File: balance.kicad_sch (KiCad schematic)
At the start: 24 parts, among them Q10 2N7002, Q5 AO3401A, Q6 AO3401A, Q7 AO3401A, Q8 2N7002, Q9 2N7002

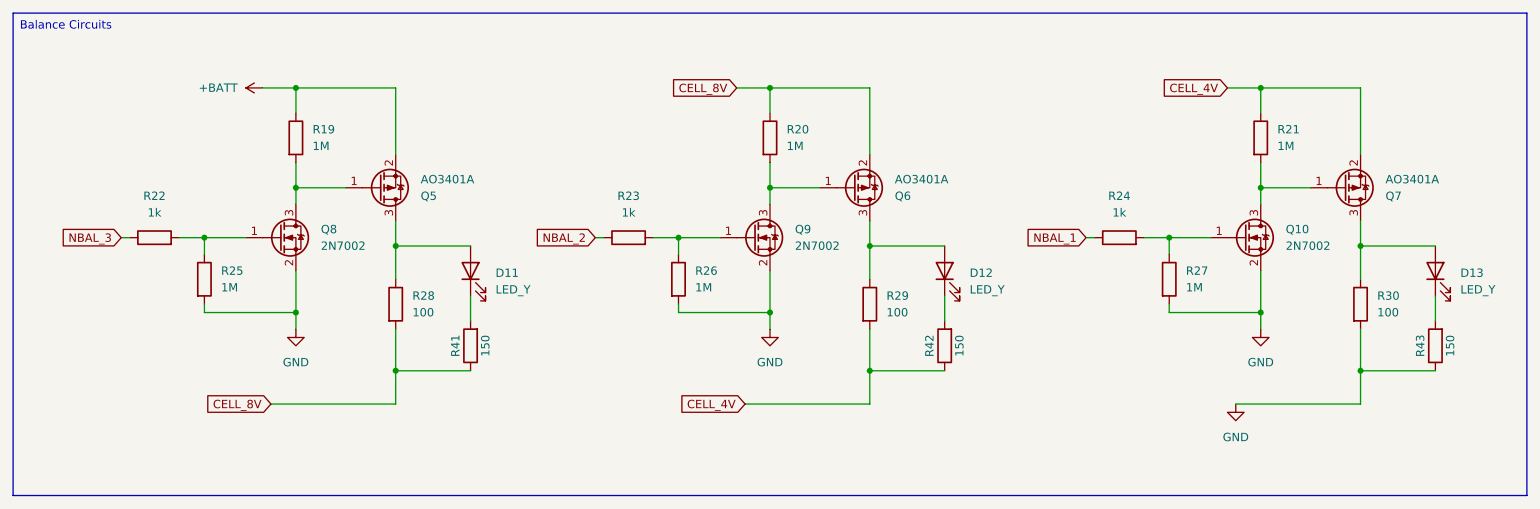
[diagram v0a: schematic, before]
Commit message: Decent pass
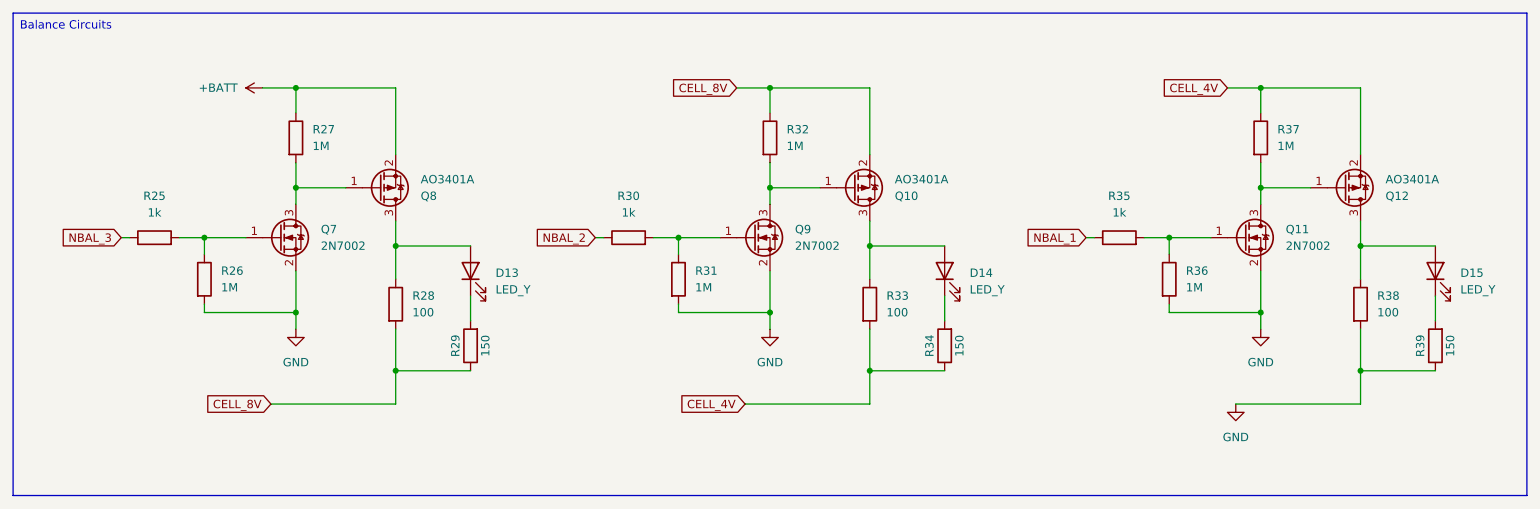
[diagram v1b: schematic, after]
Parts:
- renumbered D11 to D13, D12 to D14, D13 to D15, Q6 to Q10, Q10 to Q11, Q7 to Q12, Q8 to Q7, Q5 to Q8, R22 to R25, R25 to R26, R19 to R27, R41 to R29, R23 to R30, R26 to R31, R20 to R32, R29 to R33, R42 to R34, R24 to R35, R27 to R36, R21 to R37, R30 to R38, R43 to R39
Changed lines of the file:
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@@
 		(dnp no)
 		(fields_autoplaced yes)
-		(property "Reference" "D12"
+		(property "Reference" "D14"
 			(at 184.15 65.0874 90)
 			(effects
@@
 			(project "JPBms2"
 				(path "/d86e471c-a8be-422d-a5d1-5a4699b7b766/220685a5-608c-4c12-9441-6825efcef07c"
-					(reference "D12")
+					(reference "D14")
 					(unit 1)
 				)
@@
 		(dnp no)
 		(fields_autoplaced yes)
-		(property "Reference" "#PWR042"
+		(property "Reference" "#PWR048"
 			(at 80.01 36.83 0)
 			(effects
@@
 			(project "JPBms2"
 				(path "/d86e471c-a8be-422d-a5d1-5a4699b7b766/220685a5-608c-4c12-9441-6825efcef07c"
-					(reference "#PWR042")
+					(reference "#PWR048")
 					(unit 1)
 				)
@@
 		(dnp no)
 		(fields_autoplaced yes)
-		(property "Reference" "R25"
+		(property "Reference" "R26"
 			(at 69.85 64.7699 0)
 			(effects
@@
 			(project "JPBms2"
 				(path "/d86e471c-a8be-422d-a5d1-5a4699b7b766/220685a5-608c-4c12-9441-6825efcef07c"
-					(reference "R25")
+					(reference "R26")
 					(unit 1)
 				)
@@
 		(dnp no)
 		(fields_autoplaced yes)
-		(property "Reference" "R27"
+		(property "Reference" "R36"
 			(at 217.17 64.7699 0)
 			(effects
@@
 			(project "JPBms2"
 				(path "/d86e471c-a8be-422d-a5d1-5a4699b7b766/220685a5-608c-4c12-9441-6825efcef07c"
-					(reference "R27")
+					(reference "R36")
 					(unit 1)
 				)
@@
 		(dnp no)
 		(fields_autoplaced yes)
-		(property "Reference" "R24"
+		(property "Reference" "R35"
 			(at 207.01 53.34 90)
 			(effects
@@
 			(project "JPBms2"
 				(path "/d86e471c-a8be-422d-a5d1-5a4699b7b766/220685a5-608c-4c12-9441-6825efcef07c"
-					(reference "R24")
+					(reference "R35")
 					(unit 1)
 				)
@@
 		(on_board yes)
 		(dnp no)
-		(property "Reference" "R42"
+		(property "Reference" "R34"
 			(at 178.054 76.2 90)
 			(effects
@@
 			(project "JPBms2"
 				(path "/d86e471c-a8be-422d-a5d1-5a4699b7b766/220685a5-608c-4c12-9441-6825efcef07c"
-					(reference "R42")
+					(reference "R34")
 					(unit 1)
 				)
@@
 		(on_board yes)
 		(dnp no)
-		(property "Reference" "R43"
+		(property "Reference" "R39"
 			(at 252.984 76.2 90)
 			(effects
@@
 			(project "JPBms2"
 				(path "/d86e471c-a8be-422d-a5d1-5a4699b7b766/220685a5-608c-4c12-9441-6825efcef07c"
-					(reference "R43")
+					(reference "R39")
 					(unit 1)
 				)
@@
 		(dnp no)
 		(fields_autoplaced yes)
-		(property "Reference" "Q8"
+		(property "Reference" "Q7"
 			(at 85.09 58.4199 0)
 			(effects
@@
 			(project "JPBms2"
 				(path "/d86e471c-a8be-422d-a5d1-5a4699b7b766/220685a5-608c-4c12-9441-6825efcef07c"
-					(reference "Q8")
+					(reference "Q7")
 					(unit 1)
 				)
@@
 		(dnp no)
 		(fields_autoplaced yes)
-		(property "Reference" "R26"
+		(property "Reference" "R31"
 			(at 142.24 64.7699 0)
 			(effects
@@
 			(project "JPBms2"
 				(path "/d86e471c-a8be-422d-a5d1-5a4699b7b766/220685a5-608c-4c12-9441-6825efcef07c"
-					(reference "R26")
+					(reference "R31")
 					(unit 1)
 				)
@@
 		(on_board yes)
 		(dnp no)
-		(property "Reference" "R41"
+		(property "Reference" "R29"
 			(at 105.664 76.2 90)
 			(effects
@@
 			(project "JPBms2"
 				(path "/d86e471c-a8be-422d-a5d1-5a4699b7b766/220685a5-608c-4c12-9441-6825efcef07c"
-					(reference "R41")
+					(reference "R29")
 					(unit 1)
 				)
@@
 		(dnp no)
 		(fields_autoplaced yes)
-		(property "Reference" "R20"
+		(property "Reference" "R32"
 			(at 156.21 43.1799 0)
 			(effects
@@
 			(project "JPBms2"
 				(path "/d86e471c-a8be-422d-a5d1-5a4699b7b766/220685a5-608c-4c12-9441-6825efcef07c"
-					(reference "R20")
+					(reference "R32")
 					(unit 1)
 				)
@@
 		(dnp no)
 		(fields_autoplaced yes)
-		(property "Reference" "#PWR046"
+		(property "Reference" "#PWR051"
 			(at 224.79 91.44 0)
 			(effects
@@
 			(project "JPBms2"
 				(path "/d86e471c-a8be-422d-a5d1-5a4699b7b766/220685a5-608c-4c12-9441-6825efcef07c"
-					(reference "#PWR046")
+					(reference "#PWR051")
 					(unit 1)
 				)
@@
 		(dnp no)
 		(fields_autoplaced yes)
-		(property "Reference" "Q10"
+		(property "Reference" "Q11"
 			(at 232.41 58.4199 0)
 			(effects
@@
 			(project "JPBms2"
 				(path "/d86e471c-a8be-422d-a5d1-5a4699b7b766/220685a5-608c-4c12-9441-6825efcef07c"
-					(reference "Q10")
+					(reference "Q11")
 					(unit 1)
 				)
@@
 		(dnp no)
 		(fields_autoplaced yes)
-		(property "Reference" "R30"
+		(property "Reference" "R38"
 			(at 246.38 68.5799 0)
 			(effects
@@
 			(project "JPBms2"
 				(path "/d86e471c-a8be-422d-a5d1-5a4699b7b766/220685a5-608c-4c12-9441-6825efcef07c"
-					(reference "R30")
+					(reference "R38")
 					(unit 1)
 				)
@@
 		(dnp no)
 		(fields_autoplaced yes)
-		(property "Reference" "#PWR045"
+		(property "Reference" "#PWR052"
 			(at 228.6 80.01 0)
 			(effects
@@
 			(project "JPBms2"
 				(path "/d86e471c-a8be-422d-a5d1-5a4699b7b766/220685a5-608c-4c12-9441-6825efcef07c"
-					(reference "#PWR045")
+					(reference "#PWR052")
 					(unit 1)
 				)
@@
 		(dnp no)
 		(fields_autoplaced yes)
-		(property "Reference" "R19"
+		(property "Reference" "R27"
 			(at 83.82 43.1799 0)
 			(effects
@@
 			(project "JPBms2"
 				(path "/d86e471c-a8be-422d-a5d1-5a4699b7b766/220685a5-608c-4c12-9441-6825efcef07c"
-					(reference "R19")
+					(reference "R27")
 					(unit 1)
 				)
@@
 		(dnp no)
 		(fields_autoplaced yes)
-		(property "Reference" "R23"
+		(property "Reference" "R30"
 			(at 132.08 53.34 90)
 			(effects
@@
 			(project "JPBms2"
 				(path "/d86e471c-a8be-422d-a5d1-5a4699b7b766/220685a5-608c-4c12-9441-6825efcef07c"
-					(reference "R23")
+					(reference "R30")
 					(unit 1)
 				)
@@
 		(dnp no)
 		(fields_autoplaced yes)
-		(property "Reference" "D11"
+		(property "Reference" "D13"
 			(at 111.76 65.0874 90)
 			(effects
@@
 			(project "JPBms2"
 				(path "/d86e471c-a8be-422d-a5d1-5a4699b7b766/220685a5-608c-4c12-9441-6825efcef07c"
-					(reference "D11")
+					(reference "D13")
 					(unit 1)
 				)
@@
 		(dnp no)
 		(fields_autoplaced yes)
-		(property "Reference" "R22"
+		(property "Reference" "R25"
 			(at 59.69 53.34 90)
 			(effects
@@
 			(project "JPBms2"
 				(path "/d86e471c-a8be-422d-a5d1-5a4699b7b766/220685a5-608c-4c12-9441-6825efcef07c"
-					(reference "R22")
+					(reference "R25")
 					(unit 1)
 				)
@@
 		(dnp no)
 		(fields_autoplaced yes)
-		(property "Reference" "R29"
+		(property "Reference" "R33"
 			(at 171.45 68.5799 0)
 			(effects
@@
 			(project "JPBms2"
 				(path "/d86e471c-a8be-422d-a5d1-5a4699b7b766/220685a5-608c-4c12-9441-6825efcef07c"
-					(reference "R29")
+					(reference "R33")
 					(unit 1)
 				)
@@
 		(on_board yes)
 		(dnp no)
-		(property "Reference" "Q5"
+		(property "Reference" "Q8"
 			(at 100.33 53.3401 0)
 			(effects
@@
 			(project "JPBms2"
 				(path "/d86e471c-a8be-422d-a5d1-5a4699b7b766/220685a5-608c-4c12-9441-6825efcef07c"
-					(reference "Q5")
+					(reference "Q8")
 					(unit 1)
 				)
@@
 		(on_board yes)
 		(dnp no)
-		(property "Reference" "Q6"
+		(property "Reference" "Q10"
 			(at 172.72 53.3401 0)
 			(effects
@@
 			(project "JPBms2"
 				(path "/d86e471c-a8be-422d-a5d1-5a4699b7b766/220685a5-608c-4c12-9441-6825efcef07c"
-					(reference "Q6")
+					(reference "Q10")
 					(unit 1)
 				)
@@
 		(dnp no)
 		(fields_autoplaced yes)
-		(property "Reference" "#PWR043"
+		(property "Reference" "#PWR049"
 			(at 81.28 80.01 0)
 			(effects
@@
 			(project "JPBms2"
 				(path "/d86e471c-a8be-422d-a5d1-5a4699b7b766/220685a5-608c-4c12-9441-6825efcef07c"
-					(reference "#PWR043")
+					(reference "#PWR049")
 					(unit 1)
 				)
@@
 		(on_board yes)
 		(dnp no)
-		(property "Reference" "Q7"
+		(property "Reference" "Q12"
 			(at 247.65 53.3401 0)
 			(effects
@@
 			(project "JPBms2"
 				(path "/d86e471c-a8be-422d-a5d1-5a4699b7b766/220685a5-608c-4c12-9441-6825efcef07c"
-					(reference "Q7")
+					(reference "Q12")
 					(unit 1)
 				)
@@
 		(dnp no)
 		(fields_autoplaced yes)
-		(property "Reference" "#PWR044"
+		(property "Reference" "#PWR050"
 			(at 153.67 80.01 0)
 			(effects
@@
 			(project "JPBms2"
 				(path "/d86e471c-a8be-422d-a5d1-5a4699b7b766/220685a5-608c-4c12-9441-6825efcef07c"
-					(reference "#PWR044")
+					(reference "#PWR050")
 					(unit 1)
 				)
@@
 		(dnp no)
 		(fields_autoplaced yes)
-		(property "Reference" "D13"
+		(property "Reference" "D15"
 			(at 259.08 65.0874 90)
 			(effects
@@
 			(project "JPBms2"
 				(path "/d86e471c-a8be-422d-a5d1-5a4699b7b766/220685a5-608c-4c12-9441-6825efcef07c"
-					(reference "D13")
+					(reference "D15")
 					(unit 1)
 				)
@@
 		(dnp no)
 		(fields_autoplaced yes)
-		(property "Reference" "R21"
+		(property "Reference" "R37"
 			(at 231.14 43.1799 0)
 			(effects
@@
 			(project "JPBms2"
 				(path "/d86e471c-a8be-422d-a5d1-5a4699b7b766/220685a5-608c-4c12-9441-6825efcef07c"
-					(reference "R21")
-					(unit 1)
-				)
+					(reference "R37")
+					(unit 1)
+				)

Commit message: Routing pt1
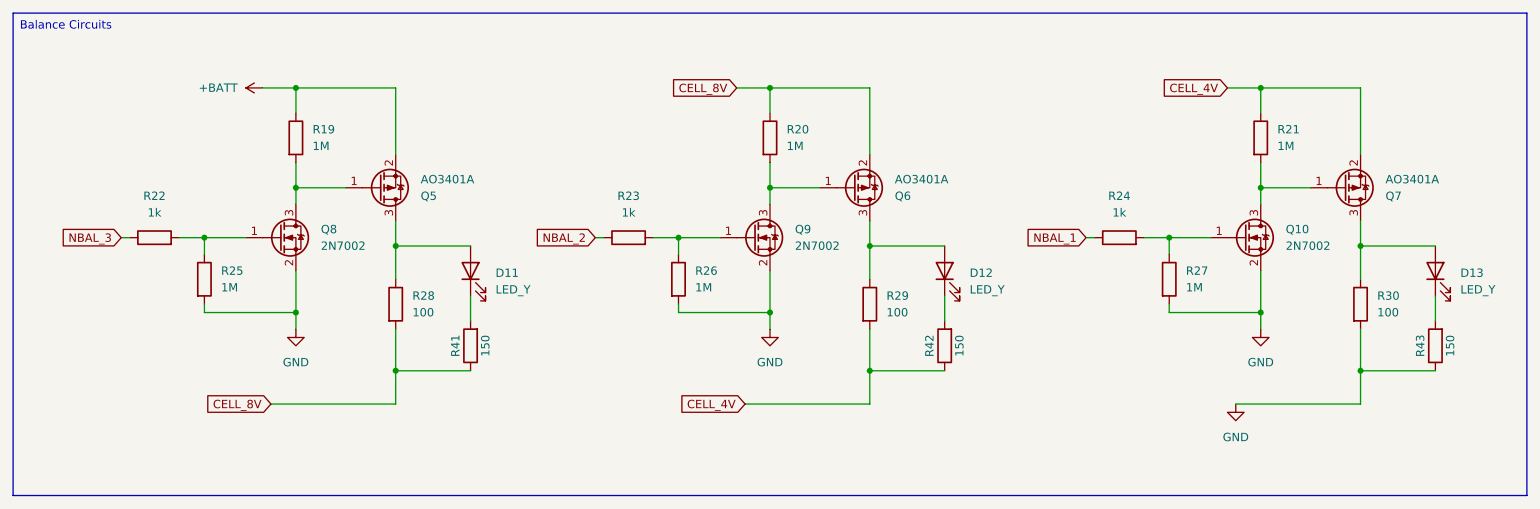
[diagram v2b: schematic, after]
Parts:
- renumbered D13 to D11, D14 to D12, D15 to D13, Q11 to Q10, Q8 to Q5, Q10 to Q6, Q12 to Q7, Q7 to Q8, R27 to R19, R32 to R20, R37 to R21, R25 to R22, R30 to R23, R35 to R24, R26 to R25, R31 to R26, R36 to R27, R33 to R29, R38 to R30, R29 to R41, R34 to R42, R39 to R43
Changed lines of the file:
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@@
 		(dnp no)
 		(fields_autoplaced yes)
-		(property "Reference" "D14"
+		(property "Reference" "D12"
 			(at 184.15 65.0874 90)
 			(effects
@@
 			(project "JPBms2"
 				(path "/d86e471c-a8be-422d-a5d1-5a4699b7b766/220685a5-608c-4c12-9441-6825efcef07c"
-					(reference "D14")
+					(reference "D12")
 					(unit 1)
 				)
@@
 		(dnp no)
 		(fields_autoplaced yes)
-		(property "Reference" "#PWR048"
+		(property "Reference" "#PWR042"
 			(at 80.01 36.83 0)
 			(effects
@@
 			(project "JPBms2"
 				(path "/d86e471c-a8be-422d-a5d1-5a4699b7b766/220685a5-608c-4c12-9441-6825efcef07c"
-					(reference "#PWR048")
+					(reference "#PWR042")
 					(unit 1)
 				)
@@
 		(dnp no)
 		(fields_autoplaced yes)
-		(property "Reference" "R26"
+		(property "Reference" "R25"
 			(at 69.85 64.7699 0)
 			(effects
@@
 			(project "JPBms2"
 				(path "/d86e471c-a8be-422d-a5d1-5a4699b7b766/220685a5-608c-4c12-9441-6825efcef07c"
-					(reference "R26")
+					(reference "R25")
 					(unit 1)
 				)
@@
 		(dnp no)
 		(fields_autoplaced yes)
-		(property "Reference" "R36"
+		(property "Reference" "R27"
 			(at 217.17 64.7699 0)
 			(effects
@@
 			(project "JPBms2"
 				(path "/d86e471c-a8be-422d-a5d1-5a4699b7b766/220685a5-608c-4c12-9441-6825efcef07c"
-					(reference "R36")
+					(reference "R27")
 					(unit 1)
 				)
@@
 		(dnp no)
 		(fields_autoplaced yes)
-		(property "Reference" "R35"
+		(property "Reference" "R24"
 			(at 207.01 53.34 90)
 			(effects
@@
 			(project "JPBms2"
 				(path "/d86e471c-a8be-422d-a5d1-5a4699b7b766/220685a5-608c-4c12-9441-6825efcef07c"
-					(reference "R35")
+					(reference "R24")
 					(unit 1)
 				)
@@
 		(on_board yes)
 		(dnp no)
-		(property "Reference" "R34"
+		(property "Reference" "R42"
 			(at 178.054 76.2 90)
 			(effects
@@
 			(project "JPBms2"
 				(path "/d86e471c-a8be-422d-a5d1-5a4699b7b766/220685a5-608c-4c12-9441-6825efcef07c"
-					(reference "R34")
+					(reference "R42")
 					(unit 1)
 				)
@@
 		(on_board yes)
 		(dnp no)
-		(property "Reference" "R39"
+		(property "Reference" "R43"
 			(at 252.984 76.2 90)
 			(effects
@@
 			(project "JPBms2"
 				(path "/d86e471c-a8be-422d-a5d1-5a4699b7b766/220685a5-608c-4c12-9441-6825efcef07c"
-					(reference "R39")
+					(reference "R43")
 					(unit 1)
 				)
@@
 		(dnp no)
 		(fields_autoplaced yes)
-		(property "Reference" "Q7"
+		(property "Reference" "Q8"
 			(at 85.09 58.4199 0)
 			(effects
@@
 			(project "JPBms2"
 				(path "/d86e471c-a8be-422d-a5d1-5a4699b7b766/220685a5-608c-4c12-9441-6825efcef07c"
-					(reference "Q7")
+					(reference "Q8")
 					(unit 1)
 				)
@@
 		(dnp no)
 		(fields_autoplaced yes)
-		(property "Reference" "R31"
+		(property "Reference" "R26"
 			(at 142.24 64.7699 0)
 			(effects
@@
 			(project "JPBms2"
 				(path "/d86e471c-a8be-422d-a5d1-5a4699b7b766/220685a5-608c-4c12-9441-6825efcef07c"
-					(reference "R31")
+					(reference "R26")
 					(unit 1)
 				)
@@
 		(on_board yes)
 		(dnp no)
-		(property "Reference" "R29"
+		(property "Reference" "R41"
 			(at 105.664 76.2 90)
 			(effects
@@
 			(project "JPBms2"
 				(path "/d86e471c-a8be-422d-a5d1-5a4699b7b766/220685a5-608c-4c12-9441-6825efcef07c"
-					(reference "R29")
+					(reference "R41")
 					(unit 1)
 				)
@@
 		(dnp no)
 		(fields_autoplaced yes)
-		(property "Reference" "R32"
+		(property "Reference" "R20"
 			(at 156.21 43.1799 0)
 			(effects
@@
 			(project "JPBms2"
 				(path "/d86e471c-a8be-422d-a5d1-5a4699b7b766/220685a5-608c-4c12-9441-6825efcef07c"
-					(reference "R32")
+					(reference "R20")
 					(unit 1)
 				)
@@
 		(dnp no)
 		(fields_autoplaced yes)
-		(property "Reference" "#PWR051"
+		(property "Reference" "#PWR046"
 			(at 224.79 91.44 0)
 			(effects
@@
 			(project "JPBms2"
 				(path "/d86e471c-a8be-422d-a5d1-5a4699b7b766/220685a5-608c-4c12-9441-6825efcef07c"
-					(reference "#PWR051")
+					(reference "#PWR046")
 					(unit 1)
 				)
@@
 		(dnp no)
 		(fields_autoplaced yes)
-		(property "Reference" "Q11"
+		(property "Reference" "Q10"
 			(at 232.41 58.4199 0)
 			(effects
@@
 			(project "JPBms2"
 				(path "/d86e471c-a8be-422d-a5d1-5a4699b7b766/220685a5-608c-4c12-9441-6825efcef07c"
-					(reference "Q11")
+					(reference "Q10")
 					(unit 1)
 				)
@@
 		(dnp no)
 		(fields_autoplaced yes)
-		(property "Reference" "R38"
+		(property "Reference" "R30"
 			(at 246.38 68.5799 0)
 			(effects
@@
 			(project "JPBms2"
 				(path "/d86e471c-a8be-422d-a5d1-5a4699b7b766/220685a5-608c-4c12-9441-6825efcef07c"
-					(reference "R38")
+					(reference "R30")
 					(unit 1)
 				)
@@
 		(dnp no)
 		(fields_autoplaced yes)
-		(property "Reference" "#PWR052"
+		(property "Reference" "#PWR045"
 			(at 228.6 80.01 0)
 			(effects
@@
 			(project "JPBms2"
 				(path "/d86e471c-a8be-422d-a5d1-5a4699b7b766/220685a5-608c-4c12-9441-6825efcef07c"
-					(reference "#PWR052")
+					(reference "#PWR045")
 					(unit 1)
 				)
@@
 		(dnp no)
 		(fields_autoplaced yes)
-		(property "Reference" "R27"
+		(property "Reference" "R19"
 			(at 83.82 43.1799 0)
 			(effects
@@
 			(project "JPBms2"
 				(path "/d86e471c-a8be-422d-a5d1-5a4699b7b766/220685a5-608c-4c12-9441-6825efcef07c"
-					(reference "R27")
+					(reference "R19")
 					(unit 1)
 				)
@@
 		(dnp no)
 		(fields_autoplaced yes)
-		(property "Reference" "R30"
+		(property "Reference" "R23"
 			(at 132.08 53.34 90)
 			(effects
@@
 			(project "JPBms2"
 				(path "/d86e471c-a8be-422d-a5d1-5a4699b7b766/220685a5-608c-4c12-9441-6825efcef07c"
-					(reference "R30")
+					(reference "R23")
 					(unit 1)
 				)
@@
 		(dnp no)
 		(fields_autoplaced yes)
-		(property "Reference" "D13"
+		(property "Reference" "D11"
 			(at 111.76 65.0874 90)
 			(effects
@@
 			(project "JPBms2"
 				(path "/d86e471c-a8be-422d-a5d1-5a4699b7b766/220685a5-608c-4c12-9441-6825efcef07c"
-					(reference "D13")
+					(reference "D11")
 					(unit 1)
 				)
@@
 		(dnp no)
 		(fields_autoplaced yes)
-		(property "Reference" "R25"
+		(property "Reference" "R22"
 			(at 59.69 53.34 90)
 			(effects
@@
 			(project "JPBms2"
 				(path "/d86e471c-a8be-422d-a5d1-5a4699b7b766/220685a5-608c-4c12-9441-6825efcef07c"
-					(reference "R25")
+					(reference "R22")
 					(unit 1)
 				)
@@
 		(dnp no)
 		(fields_autoplaced yes)
-		(property "Reference" "R33"
+		(property "Reference" "R29"
 			(at 171.45 68.5799 0)
 			(effects
@@
 			(project "JPBms2"
 				(path "/d86e471c-a8be-422d-a5d1-5a4699b7b766/220685a5-608c-4c12-9441-6825efcef07c"
-					(reference "R33")
+					(reference "R29")
 					(unit 1)
 				)
@@
 		(on_board yes)
 		(dnp no)
-		(property "Reference" "Q8"
+		(property "Reference" "Q5"
 			(at 100.33 53.3401 0)
 			(effects
@@
 			(project "JPBms2"
 				(path "/d86e471c-a8be-422d-a5d1-5a4699b7b766/220685a5-608c-4c12-9441-6825efcef07c"
-					(reference "Q8")
+					(reference "Q5")
 					(unit 1)
 				)
@@
 		(on_board yes)
 		(dnp no)
-		(property "Reference" "Q10"
+		(property "Reference" "Q6"
 			(at 172.72 53.3401 0)
 			(effects
@@
 			(project "JPBms2"
 				(path "/d86e471c-a8be-422d-a5d1-5a4699b7b766/220685a5-608c-4c12-9441-6825efcef07c"
-					(reference "Q10")
+					(reference "Q6")
 					(unit 1)
 				)
@@
 		(dnp no)
 		(fields_autoplaced yes)
-		(property "Reference" "#PWR049"
+		(property "Reference" "#PWR043"
 			(at 81.28 80.01 0)
 			(effects
@@
 			(project "JPBms2"
 				(path "/d86e471c-a8be-422d-a5d1-5a4699b7b766/220685a5-608c-4c12-9441-6825efcef07c"
-					(reference "#PWR049")
+					(reference "#PWR043")
 					(unit 1)
 				)
@@
 		(on_board yes)
 		(dnp no)
-		(property "Reference" "Q12"
+		(property "Reference" "Q7"
 			(at 247.65 53.3401 0)
 			(effects
@@
 			(project "JPBms2"
 				(path "/d86e471c-a8be-422d-a5d1-5a4699b7b766/220685a5-608c-4c12-9441-6825efcef07c"
-					(reference "Q12")
+					(reference "Q7")
 					(unit 1)
 				)
@@
 		(dnp no)
 		(fields_autoplaced yes)
-		(property "Reference" "#PWR050"
+		(property "Reference" "#PWR044"
 			(at 153.67 80.01 0)
 			(effects
@@
 			(project "JPBms2"
 				(path "/d86e471c-a8be-422d-a5d1-5a4699b7b766/220685a5-608c-4c12-9441-6825efcef07c"
-					(reference "#PWR050")
+					(reference "#PWR044")
 					(unit 1)
 				)
@@
 		(dnp no)
 		(fields_autoplaced yes)
-		(property "Reference" "D15"
+		(property "Reference" "D13"
 			(at 259.08 65.0874 90)
 			(effects
@@
 			(project "JPBms2"
 				(path "/d86e471c-a8be-422d-a5d1-5a4699b7b766/220685a5-608c-4c12-9441-6825efcef07c"
-					(reference "D15")
+					(reference "D13")
 					(unit 1)
 				)
@@
 		(dnp no)
 		(fields_autoplaced yes)
-		(property "Reference" "R37"
+		(property "Reference" "R21"
 			(at 231.14 43.1799 0)
 			(effects
@@
 			(project "JPBms2"
 				(path "/d86e471c-a8be-422d-a5d1-5a4699b7b766/220685a5-608c-4c12-9441-6825efcef07c"
-					(reference "R37")
-					(unit 1)
-				)
+					(reference "R21")
+					(unit 1)
+				)
